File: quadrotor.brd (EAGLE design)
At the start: 100 x 100 mm, 23 parts, among them T1 AO3400, T2 AO3400, T3 AO3400, T4 AO3400, X1 16MHZ

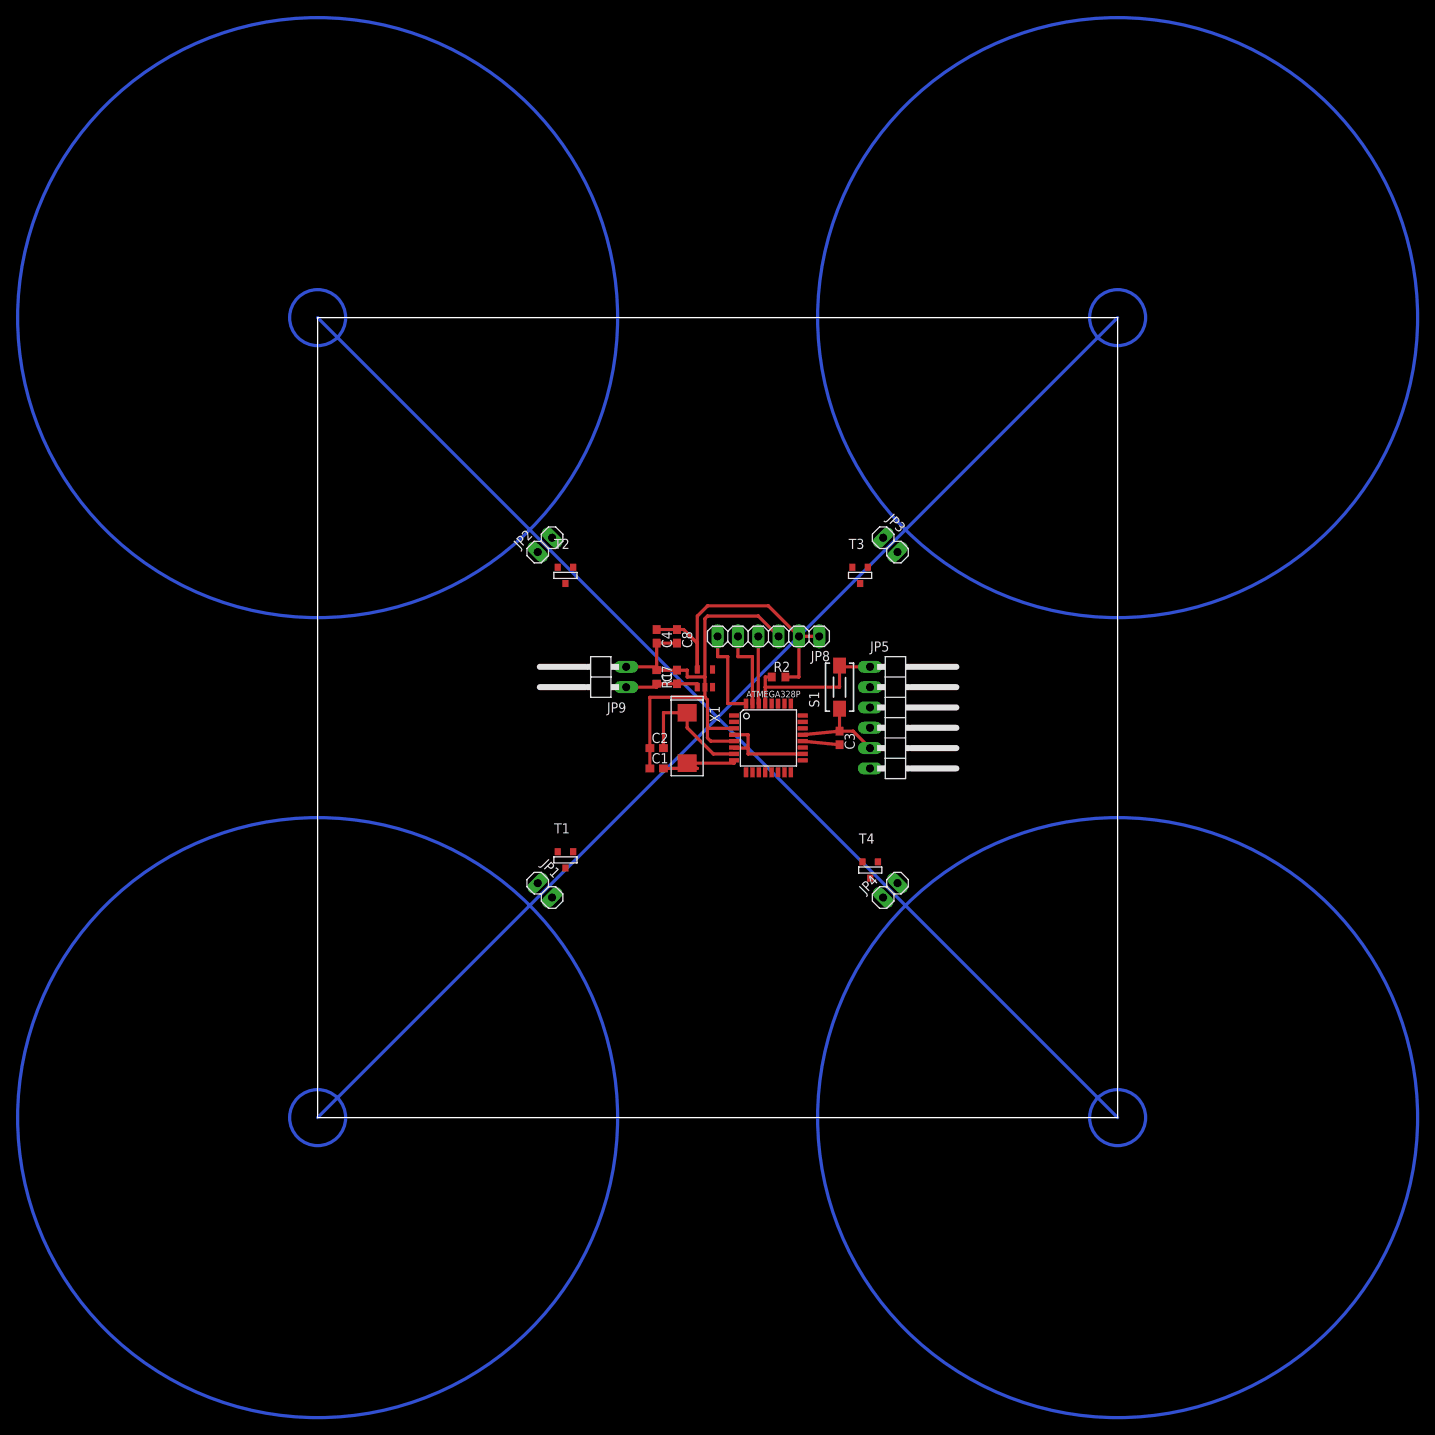
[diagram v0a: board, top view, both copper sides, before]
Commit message: mostly done layout and is routing now
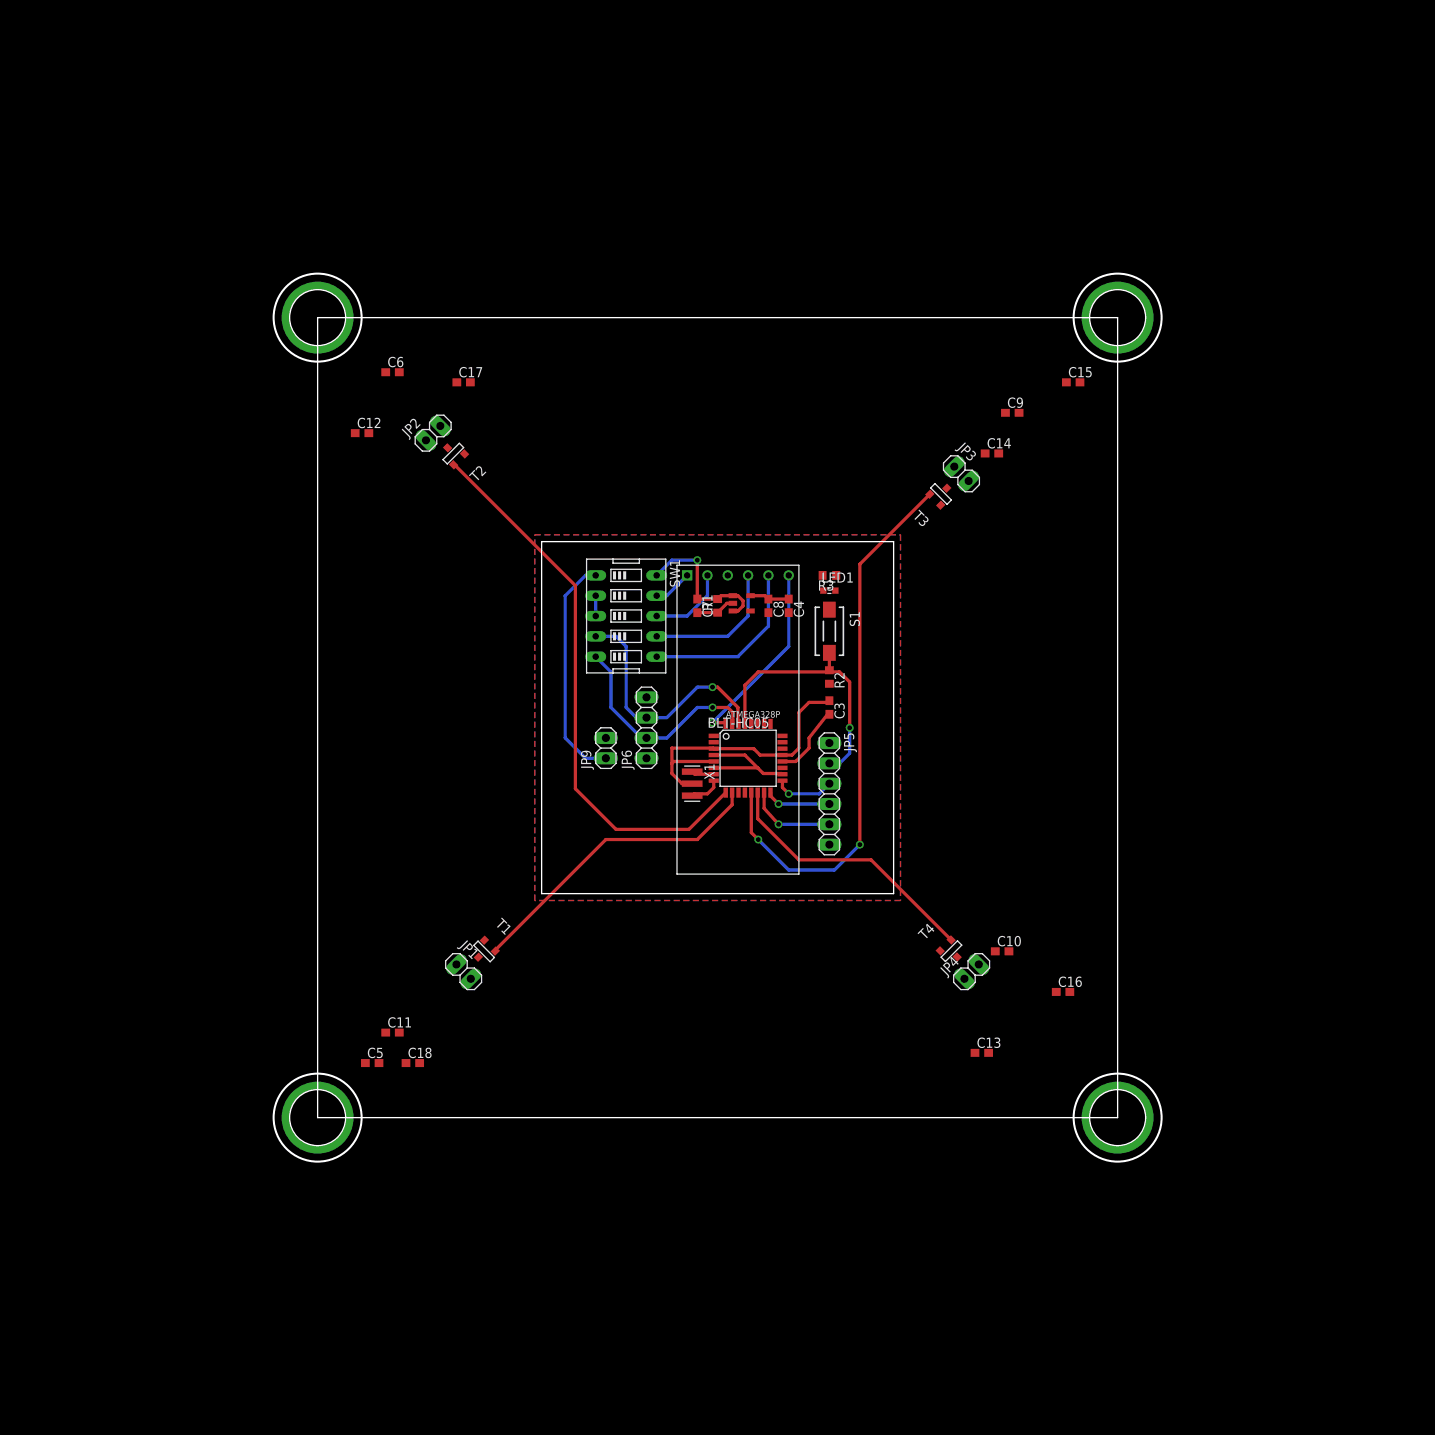
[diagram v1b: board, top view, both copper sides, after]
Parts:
- removed C1, C2: 22pF, eagle-ltspice:C0603
- removed JP8: (no value), pinhead:1X06
- added C10, C11, C12, C13, C14, C15, C16, C17, C18, C5, C6, C9: 0.1uF, eagle-ltspice:C0603
- added JP6: (no value), pinhead:1X04
- added LED1: POWER, eagle-ltspice:LED_SML0603
- added R3: 470, eagle-ltspice:R0603
- added SW1: (no value), special:EDG-05
- added U$2: BLT-HC05, quadrotor:BLT-HC05
- added U$3, U$4, U$5, U$6: 720-MSHELL, quadrotor:720MOTOR
- JP5: device pinhead:1X06/90 -> pinhead:1X06
- JP9: device pinhead:1X02/90 -> pinhead:1X02
- X1: device IQD-Frequency-Products:7.5X5-2-PAD -> murata-filter:CSTCR6M
- moved T2 20.7 mm to (-33.0, 33.0), turned to 225 degrees
- moved JP2 19.8 mm to (-35.6, 35.6)
- moved C4 16.9 mm to (8.89, 14.0)
- moved T1 15.3 mm to (-29.2, -29.2), turned to 315 degrees
- moved JP1 14.4 mm to (-31.8, -31.8)
- moved JP4 14.4 mm to (31.8, -31.8)
- moved T3 14.4 mm to (27.9, 27.9), turned to 135 degrees
- moved T4 14.4 mm to (29.2, -29.2), turned to 45 degrees
- moved JP5 13.0 mm to (14.0, -9.53)
- moved JP3 12.6 mm to (30.5, 30.5)
- moved U$1 12.3 mm to (1.91, 15.2), turned to 0 degrees
- moved C8 12.0 mm to (6.35, 14.0)
- moved R1 11.7 mm to (0.00, 14.0), turned to 90 degrees
- moved C7 9.25 mm to (-2.54, 14.0), turned to 270 degrees
- moved JP9 8.98 mm to (-14.0, -3.81)
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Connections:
- removed net PD0: ATMEGA328P.30, JP8.4
- removed net PD1: ATMEGA328P.31, JP8.5
- new net N$11: SW1.8, U$2.VCC
- new net N$12: SW1.7, U$2.TX
- new net N$13: SW1.6, U$2.RX
- new net N$14: JP9.1, SW1.1
- new net N$15: C12.2, C17.1, U$4.SHELL
- new net N$16: C13.2, C16.1, U$6.SHELL
- new net N$3: C14.2, C15.1, U$5.SHELL
- new net N$5: C11.2, C18.1, U$3.SHELL
- new net N$7: SW1.9, U$2.EN
- new net N$8: LED1.A, R3.1
- new net PD0/RX: ATMEGA328P.30, JP6.3, SW1.4
- new net PD1/TX: ATMEGA328P.31, JP6.2, SW1.5
- net GND: now also C11.1, C12.1, C13.1, C14.1, JP5.6, JP6.4, LED1.C, U$2.GND, X1.2; no longer C1.1, C2.1, JP5.5, JP8.3
- net MISO: now also JP5.4; no longer JP5.3
- net MOSI: now also JP5.5; no longer JP5.4
- net N$1: no longer C2.2
- net N$10: now also C9.1
- net N$2: now also X1.3; no longer C1.2, X1.2
- net N$4: now also C5.1
- net N$6: now also C6.1
- net N$9: now also C10.1
- net PD2: now also U$2.STATE; no longer JP8.6
- net RESET: now also JP5.2; no longer JP5.1
- net SCK: now also JP5.3; no longer JP5.2
- net VCC: now also SW1.2, SW1.3; no longer JP8.1, JP8.2
- net VIN: now also C10.2, C15.2, C16.2, C17.2, C18.2, C5.2, C6.2, C9.2, JP5.1, JP6.1, R3.2, SW1.10; no longer JP5.6, JP9.1
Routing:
- net N$5: track 141.4 -> 0.00 mm
- net N$3: track 141.4 -> 0.00 mm
- net M2: track 0.00 -> 69.7 mm
- net M3: track 0.00 -> 69.2 mm, vias 0 -> 2
- net M1: track 0.00 -> 38.8 mm
- net GND: track 77.2 -> 42.0 mm
- net M4: track 0.00 -> 33.7 mm
- net PD0/RX: track 0.00 -> 31.2 mm, vias 0 -> 1
- net VCC: track 52.7 -> 22.6 mm
- net N$14: track 0.00 -> 28.8 mm
- net PD1/TX: track 0.00 -> 27.3 mm, vias 0 -> 1
- net N$13: track 0.00 -> 21.9 mm
- net N$12: track 0.00 -> 17.6 mm
- net N$1: track 16.5 -> 2.83 mm
- net RESET: track 20.1 -> 33.6 mm, vias 0 -> 1
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- added copper zone on layer 1, net GND
- added copper zone on layer 16, net GND
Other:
- board size 100 x 100 mm -> 111 x 111 mm
